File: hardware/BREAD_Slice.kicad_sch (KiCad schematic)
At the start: 15 parts, among them J1 Conn_01x10_Female, J2 I2C_01x04

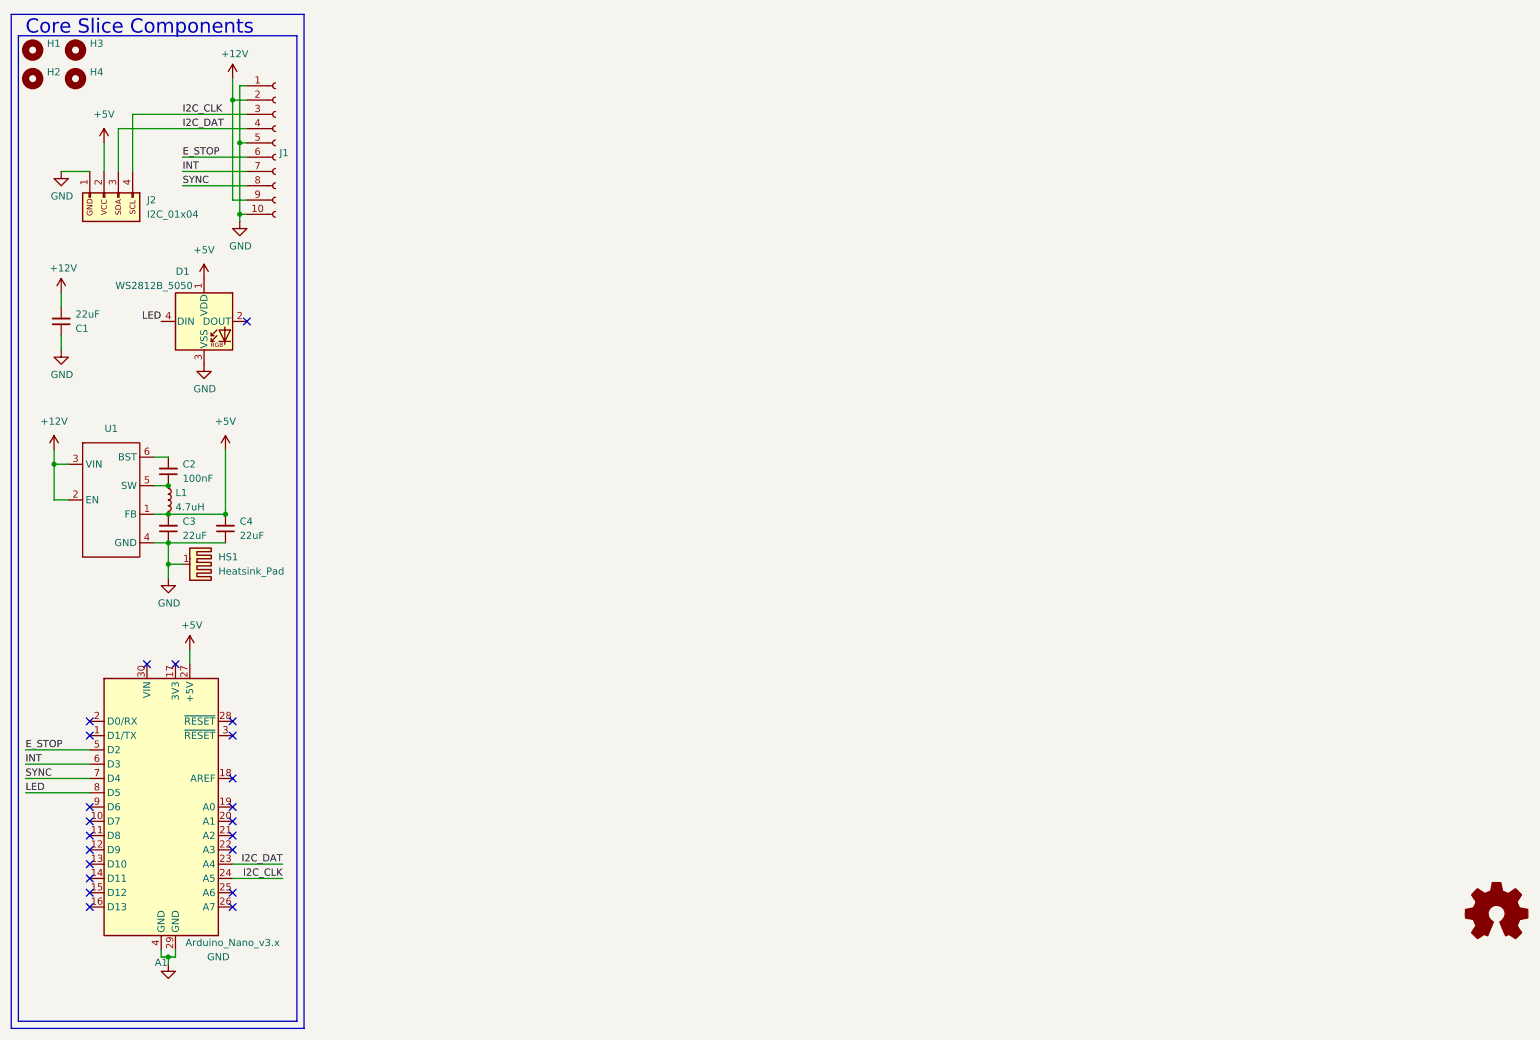
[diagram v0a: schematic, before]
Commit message: Initial commit
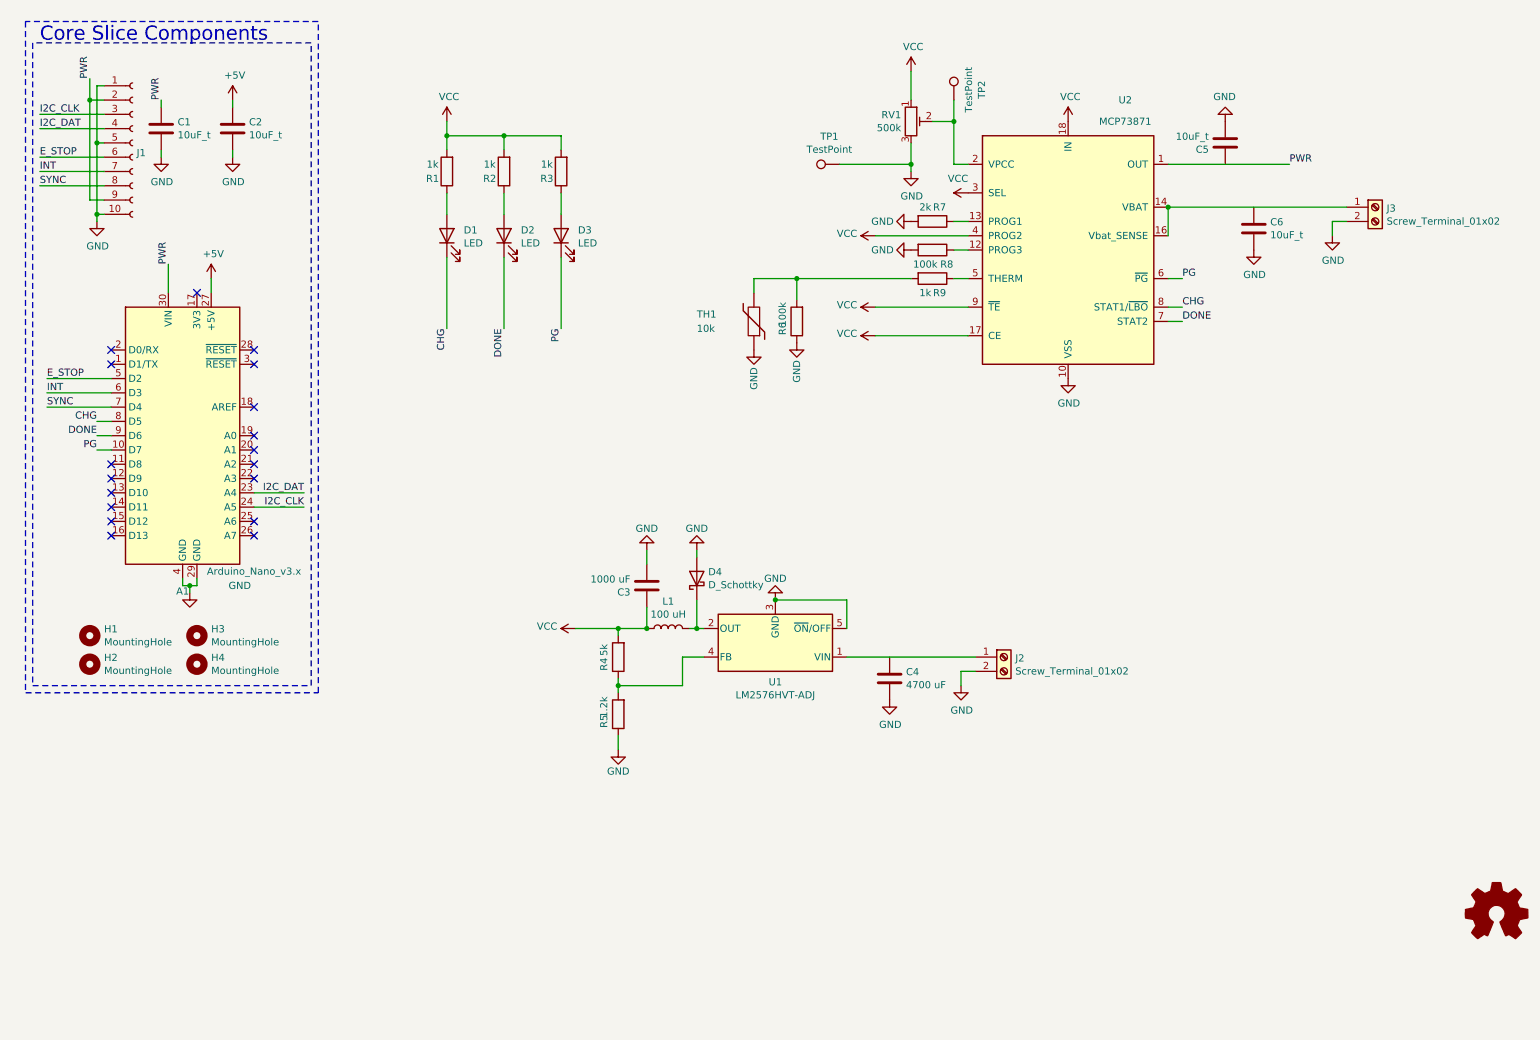
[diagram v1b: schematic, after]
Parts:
- removed C1, C3, C4: 22uF, Capacitor_SMD:C_1206_3216Metric, symbol Device:C_Small
- removed C2: 100nF, Capacitor_SMD:C_1206_3216Metric, symbol Device:C_Small
- removed D1: WS2812B_5050, SparkFun-LED:WS2812-5050-4PIN, symbol SparkFun-LED:WS2812B_5050
- removed HS1: Heatsink_Pad, SparkFun-Fuse:Thermal Pad, symbol Mechanical:Heatsink_Pad
- removed J2: I2C_01x04, Connector_JST:JST_SH_SM04B-SRSS-TB_1x04-1MP_P1.00mm_Horizontal, symbol SparkFun-Connector:I2C_01x04
- removed L1: 4.7uH, Inductor_SMD:L_1210_3225Metric, symbol Device:L_Small
- removed U1: ~, Package_TO_SOT_SMD:TSOT-23-6, symbol SparkFun-DiscreteSemi:AP63205
- added C1, C2, C5, C6: 10uF_t, OCI_UPL_FOOTPRINTS:C_2312, symbol Device:C
- added C3: 1000 uF, OCI_UPL_FOOTPRINTS:C_2312, symbol Device:C
- added C4: 4700 uF, OCI_UPL_FOOTPRINTS:C_2312, symbol Device:C
- added D1, D2, D3: LED, OCI_UPL_FOOTPRINTS:LED-5MM, symbol Device:LED
- added D4: D_Schottky, Diode_THT:D_A-405_P7.62mm_Horizontal, symbol Device:D_Schottky
- added J2, J3: Screw_Terminal_01x02, TerminalBlock_TE-Connectivity:TerminalBlock_TE_282834-2_1x02_P2.54mm_Horizontal, symbol Connector:Screw_Terminal_01x02
- added L1: 100 uH, Inductor_THT:L_Radial_D12.0mm_P10.00mm_Neosid_SD12k_style1, symbol Device:L
- added Logo1: Logo_Open_Hardware_Small, Symbol:OSHW-Symbol_6.7x6mm_SilkScreen, symbol Graphic:Logo_Open_Hardware_Small
- added R1, R2, R3, R9: 1k, OCI_UPL_FOOTPRINTS:R_1206_HandSoldering, symbol Device:R
- added R4: 5k, OCI_UPL_FOOTPRINTS:R_1206_HandSoldering, symbol Device:R
- added R5: 1.2k, OCI_UPL_FOOTPRINTS:R_1206_HandSoldering, symbol Device:R
- added R6, R8: 100k, OCI_UPL_FOOTPRINTS:R_1206_HandSoldering, symbol Device:R
- added R7: 2k, OCI_UPL_FOOTPRINTS:R_1206_HandSoldering, symbol Device:R
- added RV1: 500k, Potentiometer_THT:Potentiometer_Bourns_3296W_Vertical, symbol BREAD_Slice-rescue:R_POT_TRIM-Device
- added TH1: 10k, Resistor_THT:R_Box_L13.0mm_W4.0mm_P9.00mm, symbol Device:Thermistor
- added TP1, TP2: TestPoint, TestPoint:TestPoint_Loop_D2.54mm_Drill1.5mm_Beaded, symbol Connector:TestPoint
- added U1: LM2576HVT-ADJ, Package_TO_SOT_THT:TO-220-5_Vertical, symbol Regulator_Switching:LM2576HVT-ADJ
- added U2: MCP73871, Package_DFN_QFN:QFN-20-1EP_4x4mm_P0.5mm_EP2.5x2.5mm, symbol BREAD_Slice-rescue:MCP73871-Battery_Management
- H1, H4: footprint MountingHole:MountingHole_5mm -> MountingHole:MountingHole_3.2mm_M3_DIN965_Pad
- H2: renamed from H3; footprint MountingHole:MountingHole_5mm -> MountingHole:MountingHole_3.2mm_M3_DIN965_Pad
- H3: renamed from H2; footprint MountingHole:MountingHole_5mm -> MountingHole:MountingHole_3.2mm_M3_DIN965_Pad
- J1: symbol Connector:Conn_01x10_Female -> BREAD_Slice-rescue:Conn_01x10_Female-Connector
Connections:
- net +12V is gone; now on net PWR: J1.2 (Pin_2), J1.9 (Pin_9)
- net +5V: now also C2.1
- net GND: now also C1.2, C2.2, C3.2, C4.2, C5.2, C6.2, D4.2 (A), J2.2 (Pin_2), J3.2 (Pin_2), R5.1, R6.1, R7.2, R8.2, RV1.3, TH1.1, TP1.1, U1.3 (GND), U1.5 (~{ON}/OFF), U2.10 (VSS), U2.11 (VSS), U2.21 (VSS)
- net PG: now reaches A1.10 (D7)
- net PG: now also D3.1 (K), U2.6 (~{PG})
- net PWR: now reaches A1.30 (VIN)
- net PWR: now also C1.1, U2.1 (OUT), U2.20 (OUT)
- net DONE: now reaches A1.9 (D6)
- net DONE: now also D2.1 (K), U2.7 (STAT2)
- net LED renamed CHG
- net CHG: now also D1.1 (K), U2.8 (STAT1/~{LBO})
- new net: J3.1 (Pin_1), U2.14 (VBAT), U2.15 (VBAT), U2.16 (Vbat_SENSE)
- new net: R7.1, U2.13 (PROG1)
- new net: R6.2, R9.2, TH1.2
- new net: R8.1, U2.12 (PROG3)
- new net: D1.2 (A), R1.1
- new net: D2.2 (A), R2.1
- new net: D3.2 (A), R3.1
- new net: RV1.2, TP2.1, U2.2 (VPCC)
- new net: R9.1, U2.5 (THERM)
- new net: J2.1 (Pin_1), U1.1 (VIN)
- new net: D4.1 (K), L1.2, U1.2 (OUT)
- new net: R4.1, R5.2, U1.4 (FB)
- new net VCC: C3.1, L1.1, R1.2, R2.2, R3.2, R4.2, RV1.1, U2.17 (CE), U2.18 (IN), U2.19 (IN), U2.3 (SEL), U2.4 (PROG2), U2.9 (~{TE})
- no-connect marks 22 -> 18
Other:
- moved on the sheet: A1, H1, H2, H3, H4, J1

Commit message: finished board
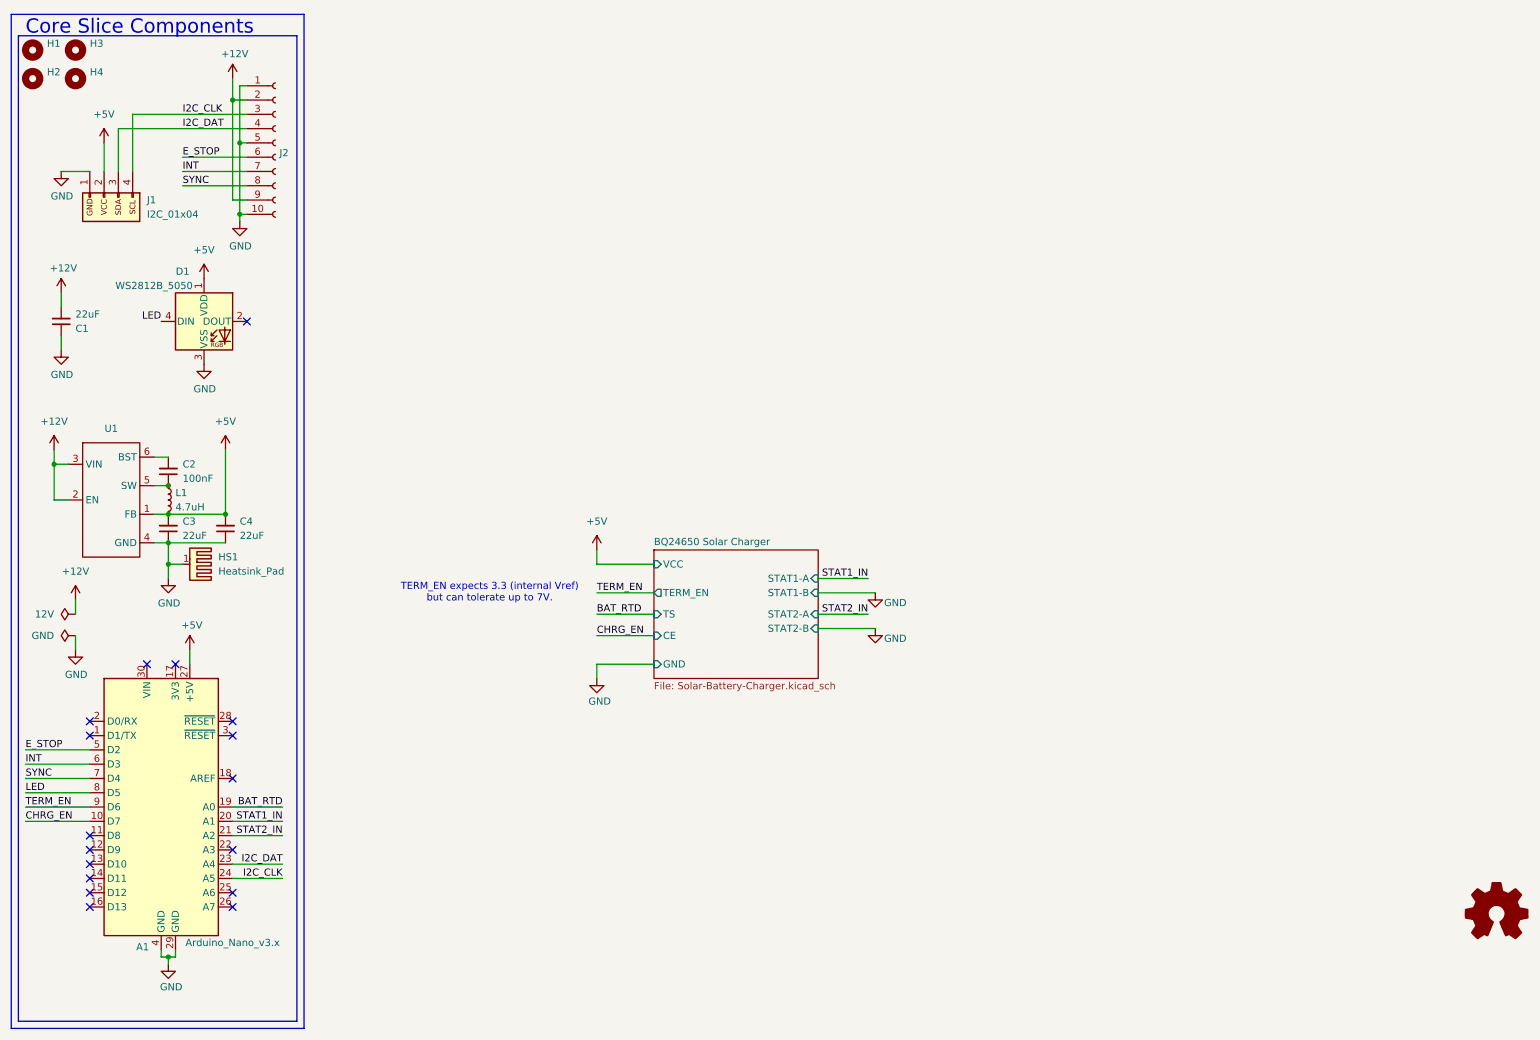
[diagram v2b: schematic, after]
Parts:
- removed C1, C2, C5, C6: 10uF_t, OCI_UPL_FOOTPRINTS:C_2312, symbol Device:C
- removed C3: 1000 uF, OCI_UPL_FOOTPRINTS:C_2312, symbol Device:C
- removed C4: 4700 uF, OCI_UPL_FOOTPRINTS:C_2312, symbol Device:C
- removed D1, D2, D3: LED, OCI_UPL_FOOTPRINTS:LED-5MM, symbol Device:LED
- removed D4: D_Schottky, Diode_THT:D_A-405_P7.62mm_Horizontal, symbol Device:D_Schottky
- removed J2, J3: Screw_Terminal_01x02, TerminalBlock_TE-Connectivity:TerminalBlock_TE_282834-2_1x02_P2.54mm_Horizontal, symbol Connector:Screw_Terminal_01x02
- removed L1: 100 uH, Inductor_THT:L_Radial_D12.0mm_P10.00mm_Neosid_SD12k_style1, symbol Device:L
- removed Logo1: Logo_Open_Hardware_Small, Symbol:OSHW-Symbol_6.7x6mm_SilkScreen, symbol Graphic:Logo_Open_Hardware_Small
- removed R1, R2, R3, R9: 1k, OCI_UPL_FOOTPRINTS:R_1206_HandSoldering, symbol Device:R
- removed R4: 5k, OCI_UPL_FOOTPRINTS:R_1206_HandSoldering, symbol Device:R
- removed R5: 1.2k, OCI_UPL_FOOTPRINTS:R_1206_HandSoldering, symbol Device:R
- removed R6, R8: 100k, OCI_UPL_FOOTPRINTS:R_1206_HandSoldering, symbol Device:R
- removed R7: 2k, OCI_UPL_FOOTPRINTS:R_1206_HandSoldering, symbol Device:R
- removed RV1: 500k, Potentiometer_THT:Potentiometer_Bourns_3296W_Vertical, symbol BREAD_Slice-rescue:R_POT_TRIM-Device
- removed TH1: 10k, Resistor_THT:R_Box_L13.0mm_W4.0mm_P9.00mm, symbol Device:Thermistor
- removed TP1, TP2: TestPoint, TestPoint:TestPoint_Loop_D2.54mm_Drill1.5mm_Beaded, symbol Connector:TestPoint
- removed U1: LM2576HVT-ADJ, Package_TO_SOT_THT:TO-220-5_Vertical, symbol Regulator_Switching:LM2576HVT-ADJ
- removed U2: MCP73871, Package_DFN_QFN:QFN-20-1EP_4x4mm_P0.5mm_EP2.5x2.5mm, symbol BREAD_Slice-rescue:MCP73871-Battery_Management
- added C1, C3, C4: 22uF, Capacitor_SMD:C_1206_3216Metric, symbol Device:C_Small
- added C2: 100nF, Capacitor_SMD:C_1206_3216Metric, symbol Device:C_Small
- added D1: WS2812B_5050, SparkFun-LED:WS2812-5050-4PIN, symbol SparkFun-LED:WS2812B_5050
- added HS1: Heatsink_Pad, KML-Custom:Thermal Pad, symbol Mechanical:Heatsink_Pad
- added J1: I2C_01x04, Connector_JST:JST_SH_SM04B-SRSS-TB_1x04-1MP_P1.00mm_Horizontal, symbol SparkFun-Connector:I2C_01x04
- added L1: 4.7uH, Inductor_SMD:L_1210_3225Metric, symbol Device:L_Small
- added U1: ~, Package_TO_SOT_SMD:TSOT-23-6, symbol SparkFun-DiscreteSemi:AP63205
- H1, H4: footprint MountingHole:MountingHole_3.2mm_M3_DIN965_Pad -> MountingHole:MountingHole_5mm
- H2: renamed from H3; footprint MountingHole:MountingHole_3.2mm_M3_DIN965_Pad -> MountingHole:MountingHole_5mm
- H3: renamed from H2; footprint MountingHole:MountingHole_3.2mm_M3_DIN965_Pad -> MountingHole:MountingHole_5mm
- J2: renamed from J1; symbol BREAD_Slice-rescue:Conn_01x10_Female-Connector -> Connector:Conn_01x10_Female
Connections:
- net +5V: now also C3.2, C4.2, D1.1 (VDD), J1.2 (Pin_2), L1.2, U1.1 (FB)
- net GND: now also C1.1, C3.1, C4.1, D1.3 (VSS), HS1.1, J1.1 (Pin_1), U1.4 (GND)
- net I2C_CLK: now also J1.4 (Pin_4)
- net I2C_DAT: now also J1.3 (Pin_3)
- net BAT_RTD: now reaches A1.19 (A0)
- net STAT1_IN: now reaches A1.20 (A1)
- net STAT2_IN: now reaches A1.21 (A2)
- net CHG renamed LED
- net LED: now also D1.4 (DIN)
- net DONE renamed TERM_EN
- net PG renamed CHRG_EN
- net PWR renamed +12V
- net +12V: now also C1.2, U1.2 (EN), U1.3 (VIN); no longer A1.30 (VIN)
- new net: C2.1, L1.1, U1.5 (SW)
- new net: C2.2, U1.6 (BST)
- no-connect marks 18 -> 17
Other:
- added sheet BQ24650 Solar Charger (Solar-Battery-Charger.kicad_sch)
- note added: "TERM_EN expects 3.3 (internal Vref) but can tolerate up to 7V."
- moved on the sheet: A1, H1, H2, H3, H4, J2
